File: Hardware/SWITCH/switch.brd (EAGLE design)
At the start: 160 x 100 mm, 4 parts, among them SW1 SWITCH-2SMD-12MM, SW2 SWITCH-2SMD-12MM

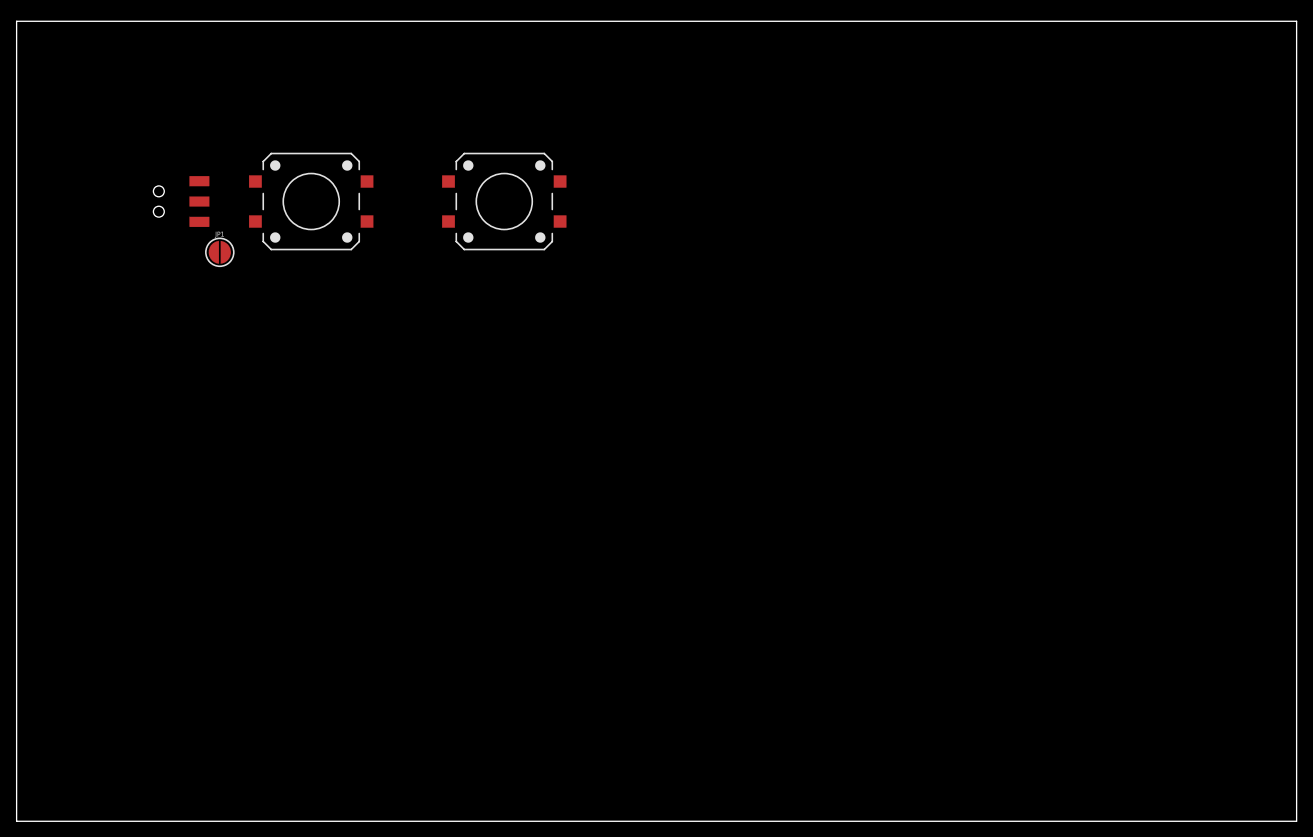
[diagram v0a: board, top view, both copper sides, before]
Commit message: update 02-10-2017
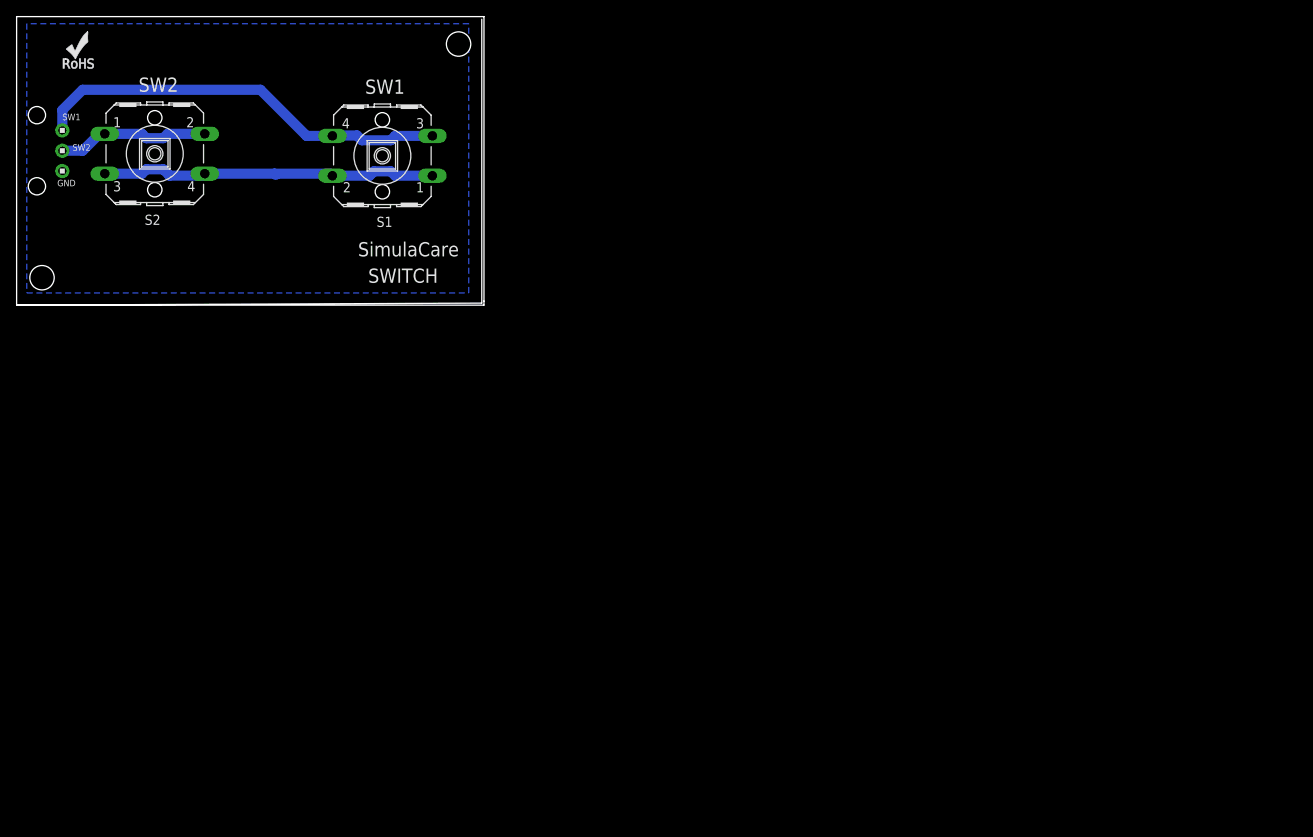
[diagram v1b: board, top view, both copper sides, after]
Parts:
- removed J1: (no value), SparkFun-Connectors:1X03_SMD_RA_MALE_POST_SMALLER
- removed JP1: (no value), SparkFun-Jumpers:SMT-JUMPER_2_NO_SILK_ROUND
- removed SW1, SW2: SWITCH-2SMD-12MM, SparkFun-Electromechanical:TACTILE-SMD-12MM
- added H1: 1X3, headers(.1in):1X3
- added S1, S2: (no value), switch-omron:B3F-40XX
- added U$1: (no value), SparkFun-Aesthetics:ROHS_LOGO_0.18_IN
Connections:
- removed net N$1: JP1.2, SW1.1, SW2.3
- net GND: now also H1.3, S1.1, S1.2, S2.3, S2.4; no longer J1.3, JP1.1
- net SW1: now also H1.1, S1.3, S1.4; no longer J1.1, SW1.3
- net SW2: now also H1.2, S2.1, S2.2; no longer J1.2, SW2.1
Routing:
- net SW1: track 0.00 -> 52.7 mm
- net GND: track 0.00 -> 42.4 mm
- net SW2: track 0.00 -> 19.1 mm
- added copper zone on layer 16, net GND
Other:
- board size 160 x 100 mm -> 58.4 x 36.1 mm
- board text added: "GND"
- board text added: "SW1"
- board text added: "SW2"
- board text added: "SWITCH"
- board text added: "SimulaCare"
